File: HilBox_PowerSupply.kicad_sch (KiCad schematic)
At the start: 63 parts, among them J13 Conn_01x10_Pin, J21 Conn_01x02_Pin, J22 Conn_01x02_Pin, J23 Conn_01x02_Pin, U29 LM5007MM, U30 LM5007MM, U31 LM5007MM

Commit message: Modification in half of target
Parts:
- J13: footprint Gascard_Lib:Terminal_Block_3_81_10p -> Connector_Phoenix_MC:PhoenixContact_MCV_1,5_10-G-3.81_1x10_P3.81mm_Vertical
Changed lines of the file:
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@@
 			)
 		)
-		(property "Footprint" "Gascard_Lib:Terminal_Block_3_81_10p"
+		(property "Footprint" "Connector_Phoenix_MC:PhoenixContact_MCV_1,5_10-G-3.81_1x10_P3.81mm_Vertical"
 			(at 19.05 39.37 0)
 			(effects

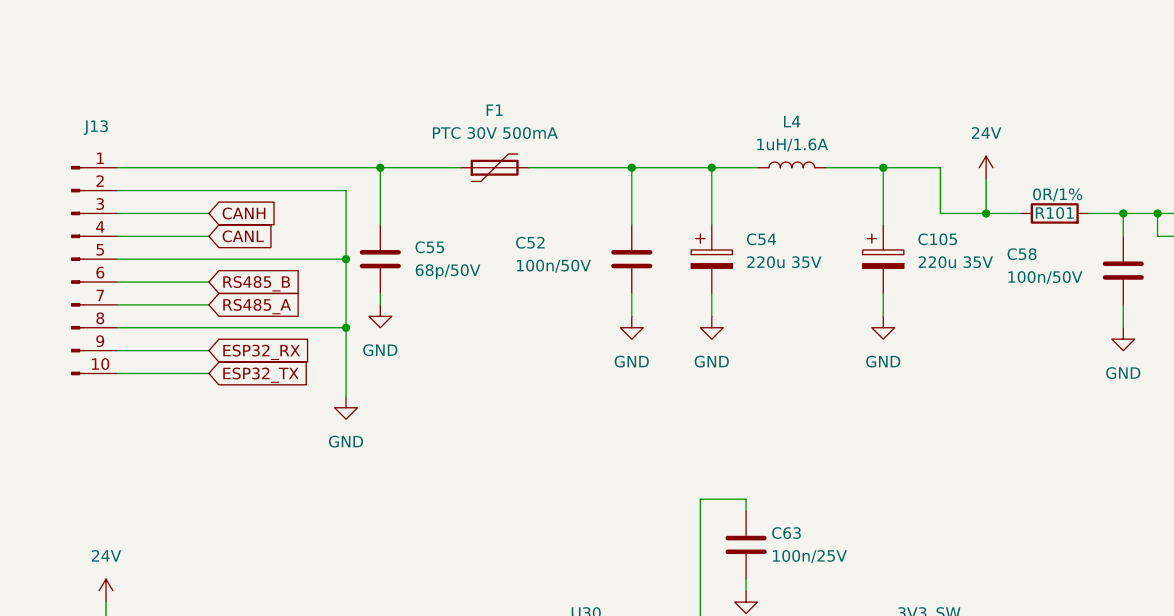
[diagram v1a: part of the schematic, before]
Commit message: Schematic design at finish
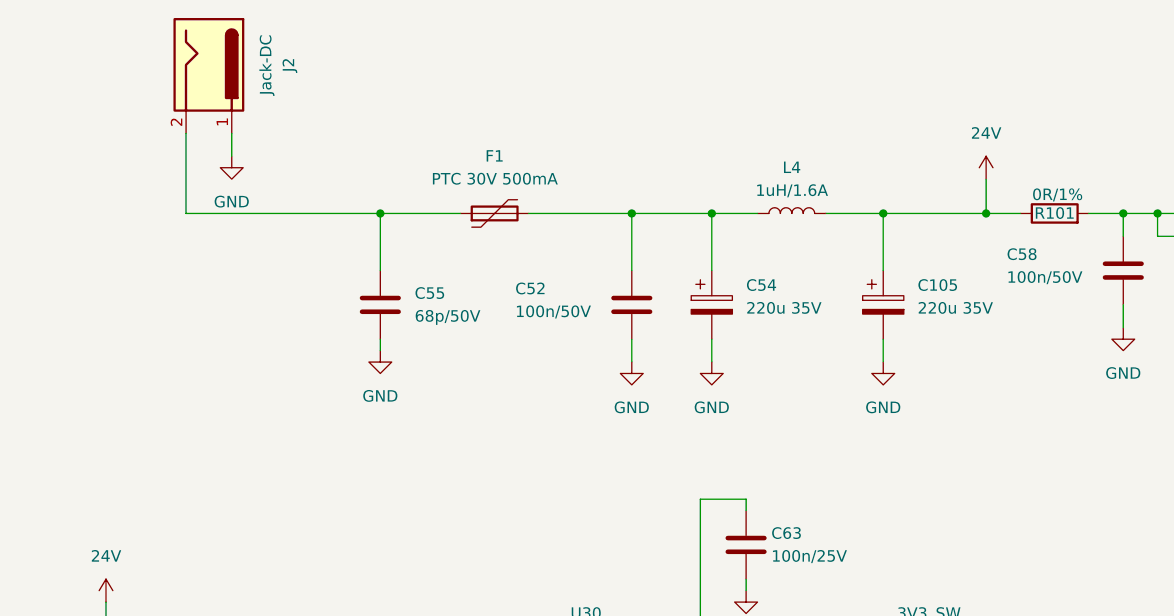
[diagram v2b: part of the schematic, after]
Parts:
- removed J13: Conn_01x10_Pin, Connector_Phoenix_MC:PhoenixContact_MCV_1,5_10-G-3.81_1x10_P3.81mm_Vertical, symbol Connector:Conn_01x10_Pin
- added J2: Jack-DC, Connector_BarrelJack:BarrelJack_GCT_DCJ200-10-A_Horizontal, symbol Connector:Jack-DC
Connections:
- net GND: now also J2.1
- net at C55.1, F1.1: now also J2.2
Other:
- moved on the sheet: C105, C52, C54, C55, F1, L4

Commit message: Layout 90% done
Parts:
- R113: footprint Resistor_SMD:R_0603_1608Metric -> Resistor_SMD:R_0402_1005Metric; JLC_PN C25804 -> C25744
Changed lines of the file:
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@@
 			)
 		)
-		(property "Footprint" "Resistor_SMD:R_0603_1608Metric"
+		(property "Footprint" "Resistor_SMD:R_0402_1005Metric"
 			(at 169.672 156.21 90)
 			(effects
@@
 			)
 		)
-		(property "JLC_PN" "C25804"
+		(property "JLC_PN" "C25744 "
 			(at 171.45 156.21 90)
 			(effects
